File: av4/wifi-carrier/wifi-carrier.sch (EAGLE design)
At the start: 12 parts, among them J1 ROCKETNET-CONNECTOR-16M, U1 UEI15

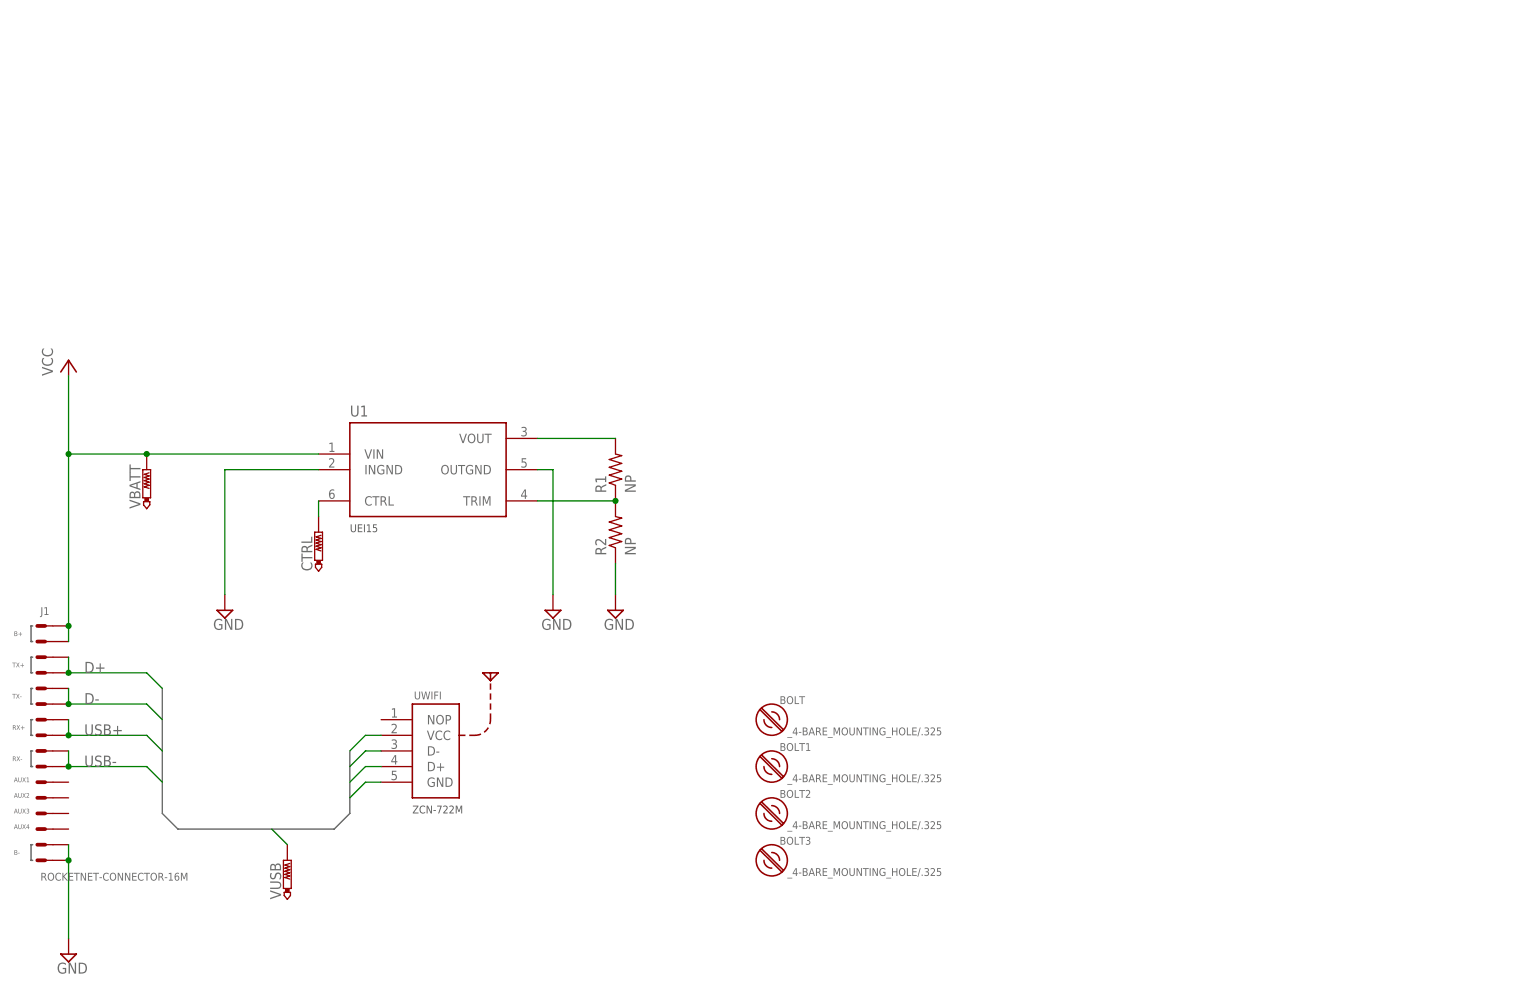
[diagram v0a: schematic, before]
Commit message: screw terminal vout
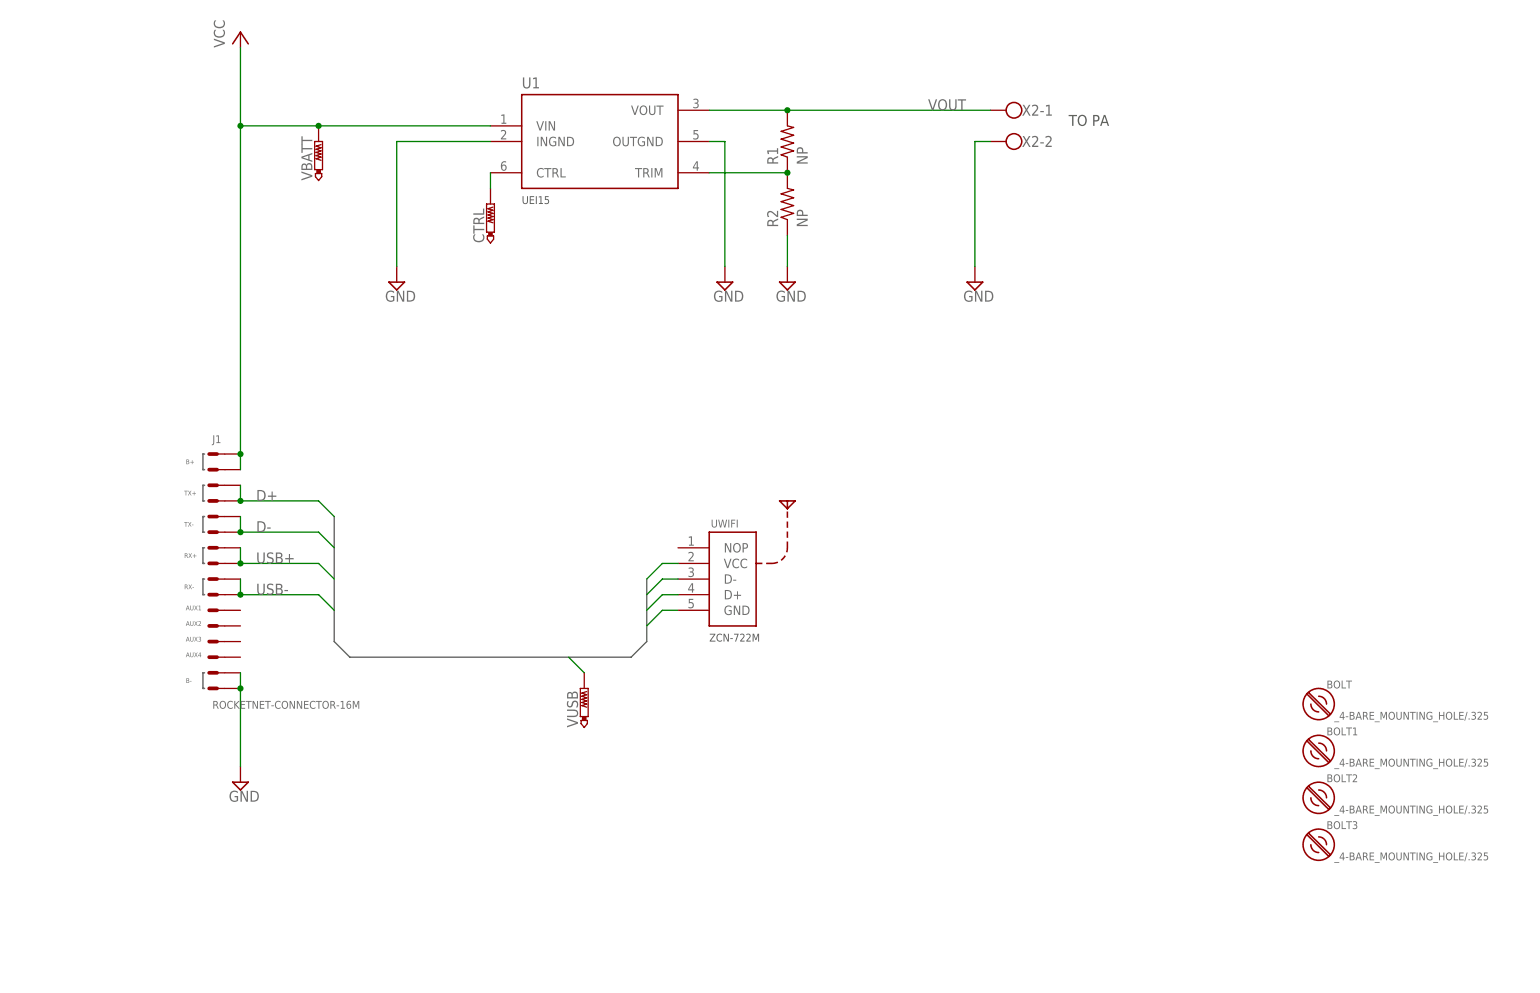
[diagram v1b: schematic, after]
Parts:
- added X2: (no value), con-wago-500:W237-102
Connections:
- net GND: now also X2-2.KL
- net VOUT: now also X2-1.KL
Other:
- note added: "TO PA"
- moved on the sheet: BOLT, BOLT1, BOLT2, BOLT3, CTRL, J1, R1, R2, U1, UWIFI, VBATT, VUSB
